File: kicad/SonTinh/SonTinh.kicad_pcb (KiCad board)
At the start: 2 copper layers, 110 x 35 mm, 9 parts, among them J8 791077010, U1 BME680, U2 TCA9517ADGK

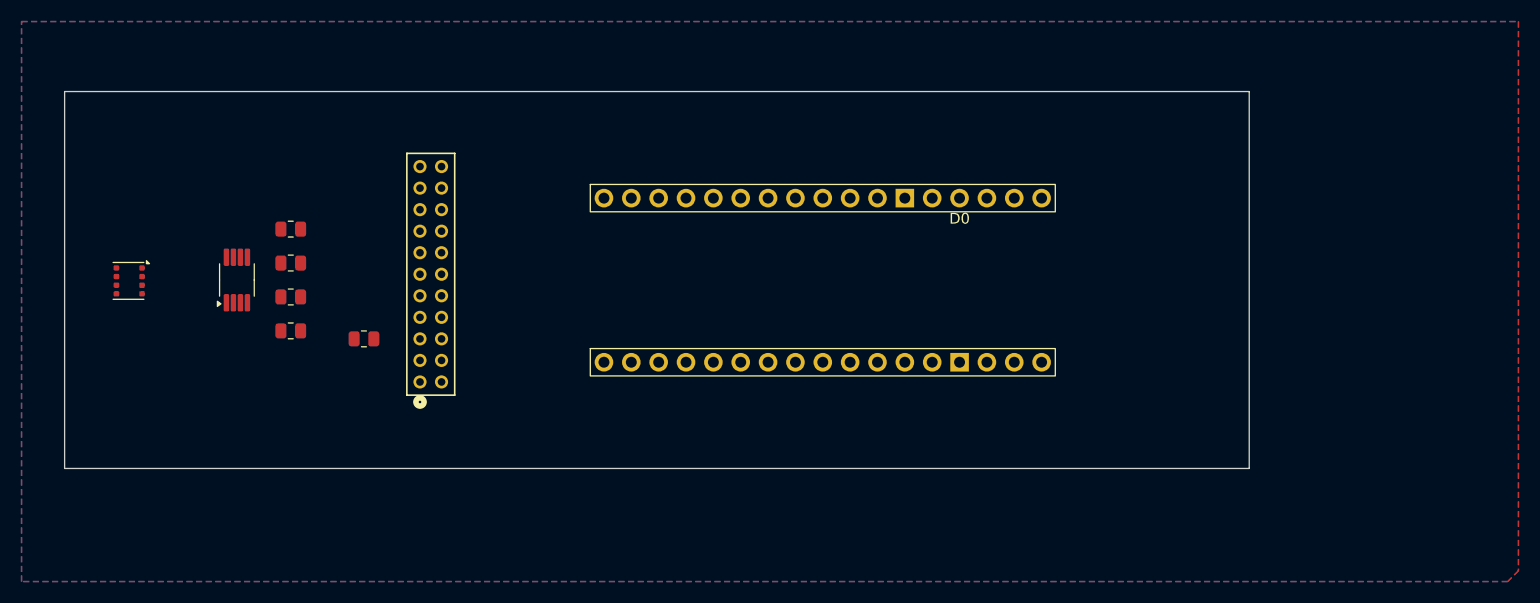
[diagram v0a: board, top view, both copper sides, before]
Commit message: A Day in the Life
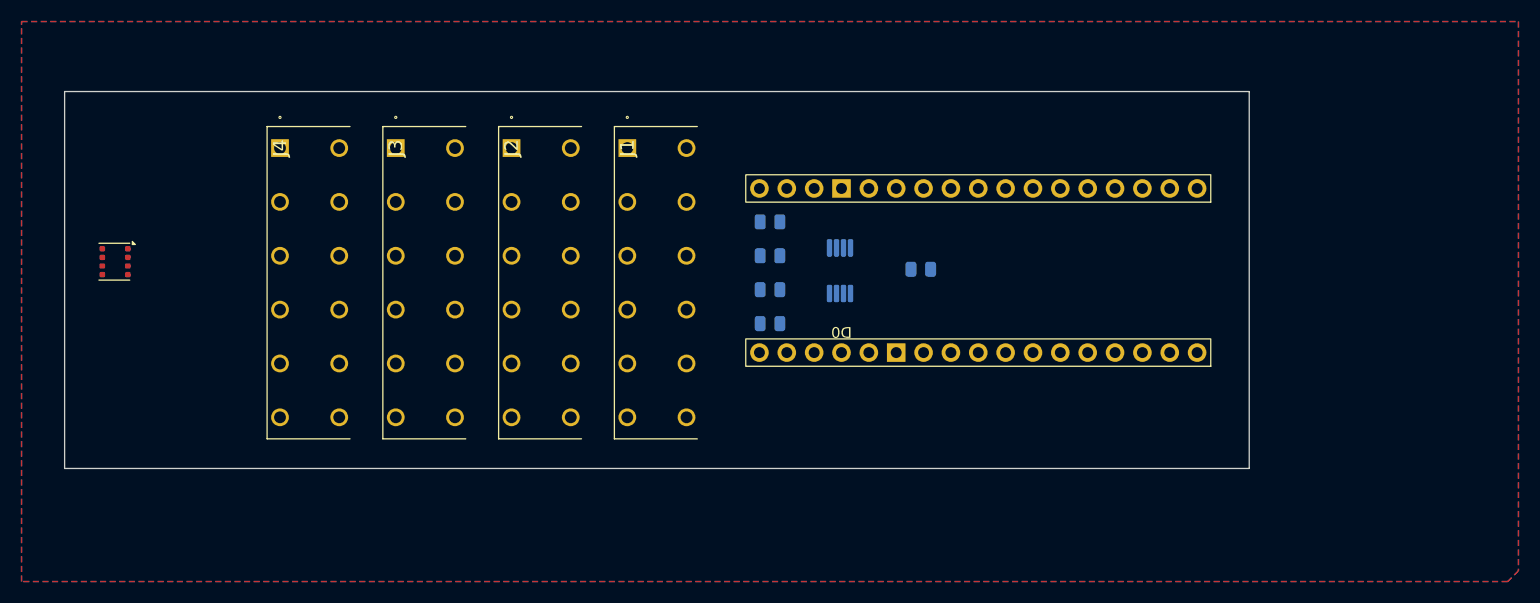
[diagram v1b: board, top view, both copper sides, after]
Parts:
- removed J8: 791077010, footprints:CONN22_791077010_MOL
- added J1: 1823450, footprints:1823450, F.Cu at (93.1, 46.7)
- added J2: 1823450, footprints:1823450, F.Cu at (82.3, 46.7)
- added J3: 1823450, footprints:1823450, F.Cu at (71.6, 46.7)
- added J4: 1823450, footprints:1823450, F.Cu at (60.8, 46.7)
- R13, R14, R15, R16, R17, U2: moved to B.Cu
- moved A1 65.7 mm to (149.9, 49.1), turned to 180 degrees
- moved U2 56.0 mm to (112.8, 58.1), turned to -90 degrees
- moved R13 52.1 mm to (120.3, 58.0)
- moved R17 45.6 mm to (106.3, 53.6)
- moved R14 45.4 mm to (106.3, 63.0)
- moved R16 44.7 mm to (106.3, 56.7)
- moved R15 44.6 mm to (106.3, 59.9)
- moved U1 2.21 mm to (45.5, 57.3)
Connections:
- A1 pad VIN: Net-(D1-K) -> +12V
